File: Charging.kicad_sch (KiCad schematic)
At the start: 20 parts, among them IC1 MP2672AGD-0000-P

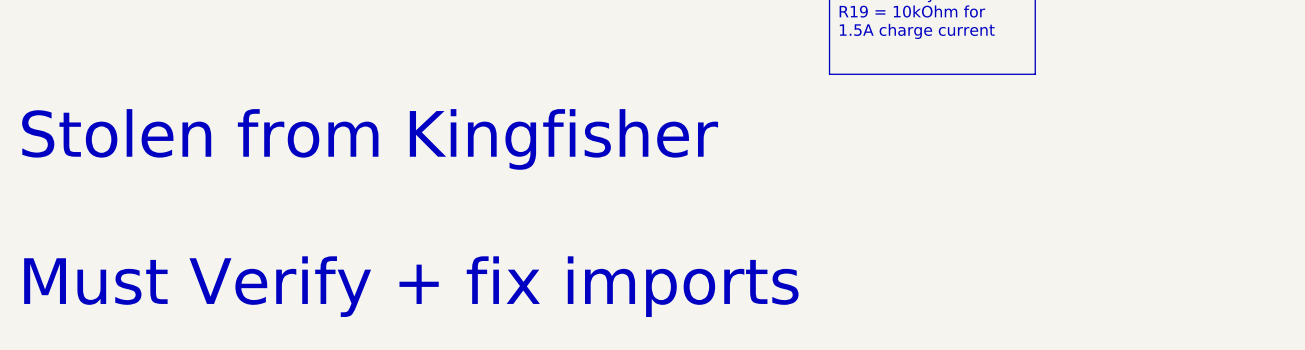
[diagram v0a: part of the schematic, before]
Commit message: Revert "Temporary save if I accidentally bust something"
This reverts commit 974f20a02fde00668d4b3d45f60811623d130148.
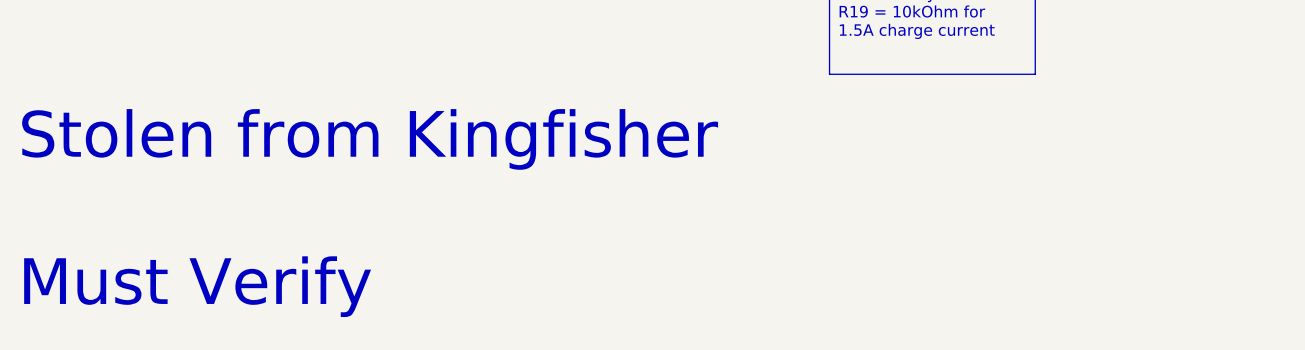
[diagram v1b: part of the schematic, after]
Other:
- note added: "Stolen from Kingfisher Must Verify"
- note removed: "Stolen from Kingfisher Must Verify + fix imports"
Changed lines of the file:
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@@
 	(generator_version "10.0")
 	(paper "A4")
-	(text "Stolen from Kingfisher\n\nMust Verify + fix imports"
+	(text "Stolen from Kingfisher\n\nMust Verify"
 		(exclude_from_sim no)
 		(at 22.86 173.99 0)

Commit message: Initial library setup
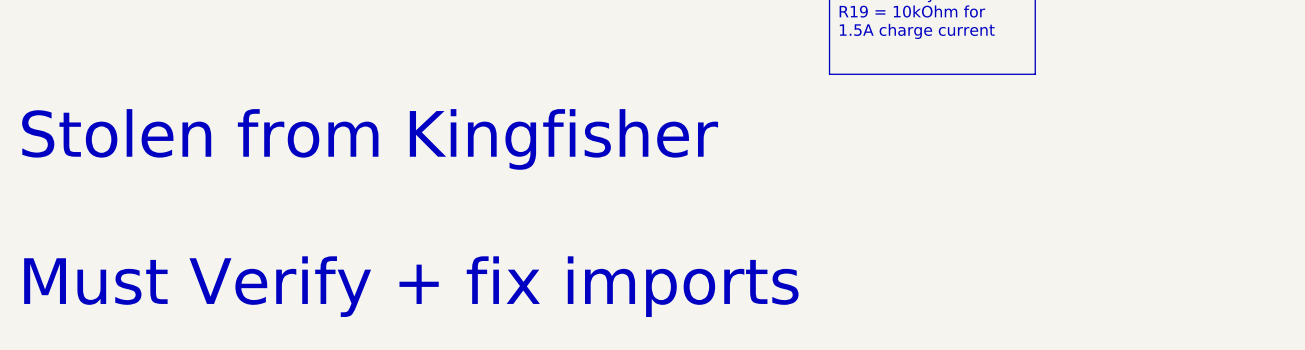
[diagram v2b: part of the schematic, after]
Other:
- note added: "Stolen from Kingfisher Must Verify + fix imports"
- note removed: "Stolen from Kingfisher Must Verify"
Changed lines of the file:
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@@
 	(generator_version "10.0")
 	(paper "A4")
-	(text "Stolen from Kingfisher\n\nMust Verify"
+	(text "Stolen from Kingfisher\n\nMust Verify + fix imports"
 		(exclude_from_sim no)
 		(at 22.86 173.99 0)
